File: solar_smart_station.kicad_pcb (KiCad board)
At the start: 6 copper layers, 46 parts, among them J1 CE, J2 CE, J3 Conn_01x03_Pin, J4 JST_VH_B2P_3.96mm, J5 JST_VH_B2P_3.96mm, J6 JST_VH_B3P_3.96mm, U1 BQ25672RQMR, U2 TLV73333PDBV, U3 MSPM0C1104SDSGR

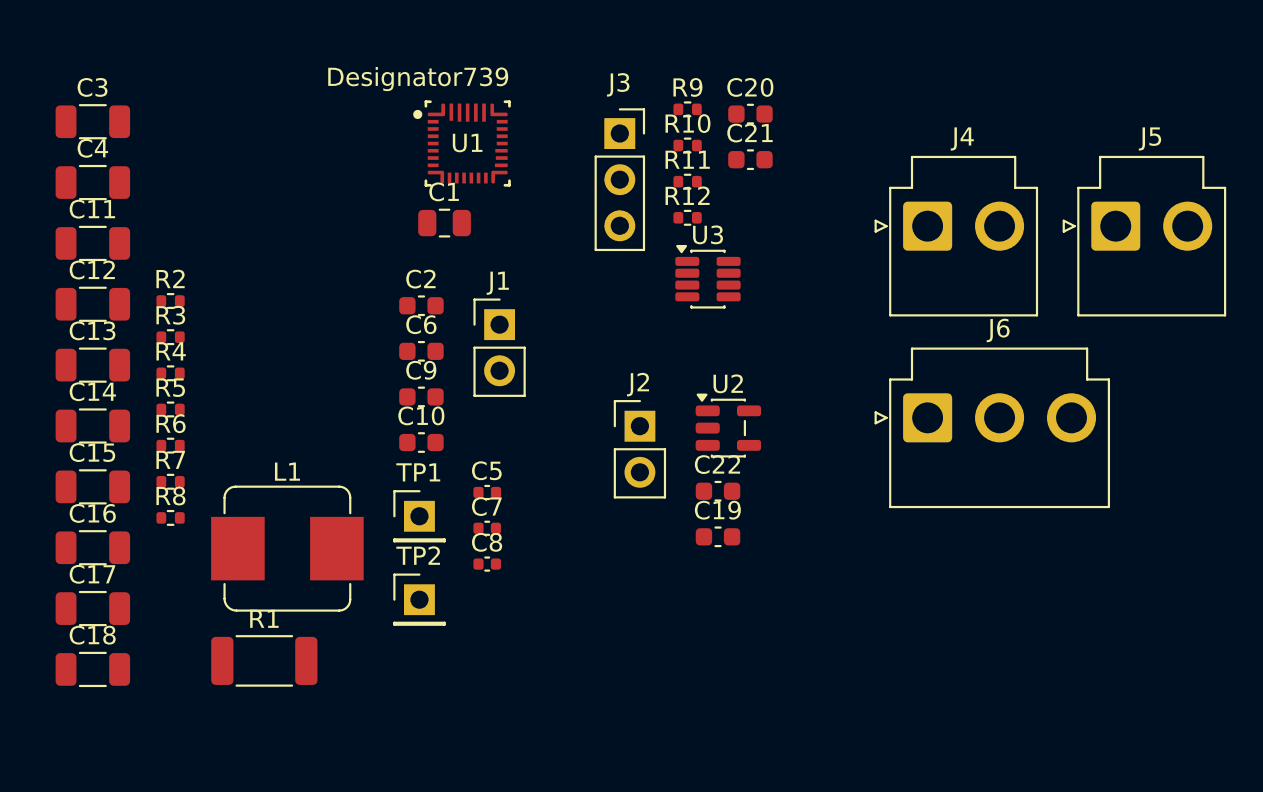
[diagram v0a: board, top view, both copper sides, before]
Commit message: First layout
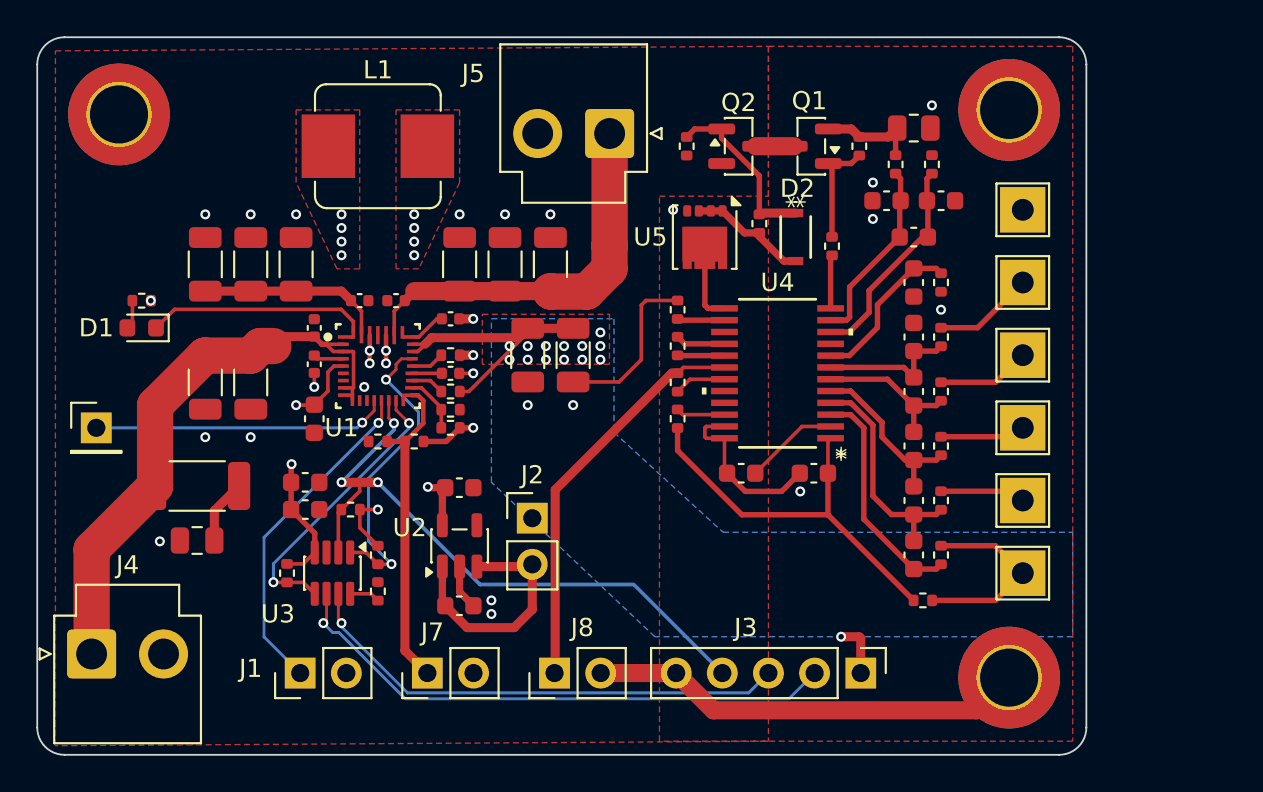
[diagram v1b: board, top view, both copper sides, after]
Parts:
- removed J6: JST_VH_B3P_3.96mm, Connector_JST:JST_VH_B3P-VH_1x03_P3.96mm_Vertical
- removed TP2: Thermistor, Connector_PinHeader_2.54mm:PinHeader_1x01_P2.54mm_Vertical
- added C23: 0.1uF, Capacitor_SMD:C_0603_1608Metric, F.Cu at (78.0, 174.5)
- added C24: 0.1uF, Capacitor_SMD:C_0603_1608Metric, F.Cu at (78.0, 171.5)
- added C25: 0.1uF, Capacitor_SMD:C_0603_1608Metric, F.Cu at (78.0, 168.5)
- added C26: 0.1uF, Capacitor_SMD:C_0603_1608Metric, F.Cu at (78.0, 165.5)
- added C27: 0.1uF, Capacitor_SMD:C_0603_1608Metric, F.Cu at (78.0, 162.5)
- added C28: 0.1uF, Capacitor_SMD:C_0603_1608Metric, F.Cu at (78.0, 159.5)
- added C29: 1uF, Capacitor_SMD:C_0603_1608Metric, F.Cu at (72.5, 170.0)
- added C30: 1uF, Capacitor_SMD:C_0603_1608Metric, F.Cu at (68.5, 170.0)
- added C31: 0.1uF, Capacitor_SMD:C_0603_1608Metric, F.Cu at (78.0, 157.0)
- added C32: 0.1uF, Capacitor_SMD:C_0603_1608Metric, F.Cu at (76.5, 155.0)
- added C33: 0.1uF, Capacitor_SMD:C_0603_1608Metric, F.Cu at (79.5, 155.0)
- added D1: LED, LED_SMD:LED_0603_1608Metric, F.Cu at (35.5, 162.0)
- added D2: Schottky_30V_1A, solar_station:DIO_RB02_ROM, F.Cu at (71.5, 157.0)
- added H1: MountingHole_Pad, TestPoint:TestPoint_THTPad_2.5x2.5mm_Drill1.2mm, F.Cu at (84.0, 175.5)
- added H2: MountingHole_Pad, TestPoint:TestPoint_THTPad_2.5x2.5mm_Drill1.2mm, F.Cu at (84.0, 171.5)
- added H3: MountingHole_Pad, TestPoint:TestPoint_THTPad_2.5x2.5mm_Drill1.2mm, F.Cu at (84.0, 167.5)
- added H4: MountingHole_Pad, TestPoint:TestPoint_THTPad_2.5x2.5mm_Drill1.2mm, F.Cu at (84.0, 163.5)
- added H5: MountingHole_Pad, TestPoint:TestPoint_THTPad_2.5x2.5mm_Drill1.2mm, F.Cu at (84.0, 159.5)
- added H6: MountingHole_Pad, TestPoint:TestPoint_THTPad_2.5x2.5mm_Drill1.2mm, F.Cu at (84.0, 155.5)
- added H7: MountingHole_Pad, MountingHole:MountingHole_3.2mm_M3_DIN965_Pad_TopBottom, F.Cu at (34.2, 150.2)
- added H8: MountingHole_Pad, MountingHole:MountingHole_3.2mm_M3_DIN965_Pad_TopBottom, F.Cu at (83.2, 150.0)
- added H9: MountingHole_Pad, MountingHole:MountingHole_3.2mm_M3_DIN965_Pad_TopBottom, F.Cu at (83.2, 181.2)
- added J7: Thermistor_1, Connector_PinHeader_2.54mm:PinHeader_1x02_P2.54mm_Vertical, F.Cu at (51.2, 181.0)
- added J8: Thermistor_2, Connector_PinHeader_2.54mm:PinHeader_1x02_P2.54mm_Vertical, F.Cu at (58.2, 181.0)
- added NT1: NetTie_3, NetTie:NetTie-3_SMD_Pad0.5mm, F.Cu at (47.5, 170.5)
- added NT2: NetTie_2, NetTie:NetTie-2_SMD_Pad0.5mm, F.Cu at (74.5, 179.0)
- added Q1: AO3400A, Package_TO_SOT_SMD:SOT-23, F.Cu at (72.4, 152.0)
- added Q2: AO3400A, Package_TO_SOT_SMD:SOT-23, F.Cu at (68.4, 152.0)
- added R13: 1kR, Resistor_SMD:R_0402_1005Metric, F.Cu at (79.5, 174.5)
- added R14: 1kR, Resistor_SMD:R_0402_1005Metric, F.Cu at (79.5, 171.5)
- added R15: 1kR, Resistor_SMD:R_0402_1005Metric, F.Cu at (79.5, 168.5)
- added R16: 1kR, Resistor_SMD:R_0402_1005Metric, F.Cu at (79.5, 165.5)
- added R17: 1kR, Resistor_SMD:R_0402_1005Metric, F.Cu at (79.5, 162.5)
- added R18: 1kR, Resistor_SMD:R_0402_1005Metric, F.Cu at (79.5, 159.5)
- added R19: 1kR, Resistor_SMD:R_0402_1005Metric, F.Cu at (78.5, 177.0)
- added R20: 100R, Resistor_SMD:R_0402_1005Metric, F.Cu at (79.0, 153.0)
- added R21: 10mR, Resistor_SMD:R_0805_2012Metric, F.Cu at (78.0, 151.0)
- added R22: 100R, Resistor_SMD:R_0402_1005Metric, F.Cu at (77.0, 153.0)
- added R23: 4.7kR, Resistor_SMD:R_0402_1005Metric, F.Cu at (73.5, 157.5)
- added R24: 1MegR, Resistor_SMD:R_0402_1005Metric, F.Cu at (75.0, 152.0)
- added R25: 1MegR, Resistor_SMD:R_0402_1005Metric, F.Cu at (69.5, 156.3)
- added R26: 3.3MegR, Resistor_SMD:R_0402_1005Metric, F.Cu at (65.5, 152.0)
- added R27: 10kR, Resistor_SMD:R_0402_1005Metric, F.Cu at (65.0, 167.0)
- added R28: 100kR, Resistor_SMD:R_0402_1005Metric, F.Cu at (65.0, 163.0)
- added R29: 450kR, Resistor_SMD:R_0402_1005Metric, F.Cu at (65.0, 161.0)
- added R30: 10kR, Resistor_SMD:R_0402_1005Metric, F.Cu at (65.0, 165.0)
- added U4: BQ7791500PWR, solar_station:PW24_TEX, F.Cu at (70.5, 164.5)
- added U5: CSD25402Q3A, Package_SON:VSON-8_3.3x3.3mm_P0.65mm_NexFET, F.Cu at (66.5, 157.0)
- C10, C2, C9: footprint Capacitor_SMD:C_0603_1608Metric -> Capacitor_SMD:C_0402_1005Metric
- J2: value CE -> LDO_EN
- J3: value Conn_01x03_Pin -> Conn_01x05_Pin; footprint Connector_PinSocket_2.54mm:PinSocket_1x03_P2.54mm_Vertical -> Connector_PinHeader_2.54mm:PinHeader_1x05_P2.54mm_Vertical
- U3: footprint Package_TO_SOT_SMD:TSOT-23-8 -> solar_station:TSOT-23-8-shrink
- moved J4 51.7 mm to (32.7, 179.9)
- moved C18 33.6 mm to (58.0, 158.5), turned to -90 degrees
- moved J3 32.5 mm to (75.1, 181.0), turned to -90 degrees
- moved C21 31.8 mm to (44.5, 170.5), turned to 180 degrees
- moved C22 31.2 mm to (44.5, 172.0), turned to 180 degrees
- moved R12 29.5 mm to (43.5, 175.5), turned to 90 degrees
- moved R9 28.8 mm to (47.0, 172.0), turned to 180 degrees
- moved J5 28.3 mm to (61.3, 151.3), turned to 180 degrees
- moved R11 28.3 mm to (48.5, 176.5), turned to 90 degrees
- moved R10 28.3 mm to (48.5, 174.5), turned to -90 degrees
- moved C16 27.5 mm to (55.5, 158.5), turned to -90 degrees
- moved C14 26.7 mm to (59.2, 163.5), turned to 90 degrees
- moved U3 26.3 mm to (46.0, 175.5), turned to -90 degrees
- moved C11 24.7 mm to (56.8, 163.5), turned to 90 degrees
- moved L1 22.7 mm to (48.5, 152.0)
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- renumbered C22 to C20, C20 to C21, C21 to C22
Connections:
- net +12V renamed +21V
- net Net-(J1-Pin_1) renamed CE_N
- net Net-(J2-Pin_2) renamed LDO_IN
- net Net-(J3-Pin_2) renamed SWDIO
- net Net-(J3-Pin_3) renamed SWCLK
- J3 pad 1: /Project Architecture/MCU/SCL -> VCC
- R10 pad 2: /Project Architecture/MCU/INT_N -> INT_N
- R12 pad 1: /Project Architecture/MCU/SDA -> SDA
- R9 pad 2: /Project Architecture/MCU/SCL -> /Project Architecture/MCU/SCL/RST
- U1 pad 14: /Project Architecture/SolarCharger/SCL -> SCL
- U1 pad 15: /Project Architecture/SolarCharger/SDA -> SDA
- U1 pad 21: /Project Architecture/SolarCharger/INT_N -> INT_N
- U3 pad 1: /Project Architecture/MCU/INT_N -> INT_N
- U3 pad 2: /Project Architecture/MCU/SCL -> /Project Architecture/MCU/SCL/RST
- U3 pad 5: /Project Architecture/MCU/SDA -> SDA
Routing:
- net +3V3: track 0.00 -> 51.2 mm, vias 0 -> 4
- net GND: track 0.00 -> 37.4 mm, vias 0 -> 16
- net REGN: track 0.00 -> 34.1 mm, vias 0 -> 3
- net +21V: track 0.00 -> 32.3 mm
- net SWDIO: track 0.00 -> 31.0 mm, vias 0 -> 1
- net SWCLK: track 0.00 -> 27.3 mm, vias 0 -> 1
- net BATTERY_PACK: track 0.00 -> 26.1 mm, vias 0 -> 13
- net RST: track 0.00 -> 23.3 mm, vias 0 -> 1
- net THERMISTOR_2: track 0.00 -> 22.2 mm
- net Net-(U4-VDD): track 0.00 -> 21.9 mm
- net SYSTEM_LOAD: track 0.00 -> 21.6 mm
- net CE_N: track 0.00 -> 18.5 mm, vias 0 -> 1
- net THERMISTOR: track 0.00 -> 18.3 mm
- net INT_N: track 0.00 -> 17.2 mm, vias 0 -> 2
- net Net-(U1-SW2): track 0.00 -> 16.7 mm, vias 0 -> 7
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- added copper zone on F.Cu, net -BATT
- added copper zone on In1.Cu, net -BATT
- added copper zone on B.Cu, net BATTERY_PACK
- added copper zone on F.Cu, net BATTERY_PACK
- added copper zone on F.Cu, net GND
- added copper zone on In1.Cu, net GND
- added copper zone on F.Cu, net Net-(U1-SW1)
- added copper zone on F.Cu, net Net-(U1-SW2)
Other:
- board outline added: 57.8 x 39.5 mm
- copper layers 6 -> 4
